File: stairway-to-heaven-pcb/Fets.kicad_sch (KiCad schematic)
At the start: 7 parts, among them J14 Conn_01x04_Male, Q40 FDN337N, Q41 FDN337N, Q42 FDN337N

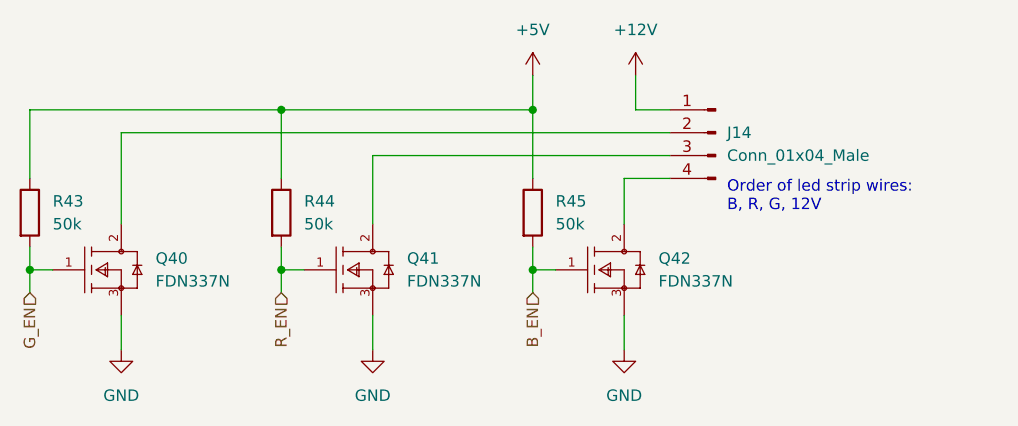
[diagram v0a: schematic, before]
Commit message: Change to 4 layer pcb. Routing leds done.
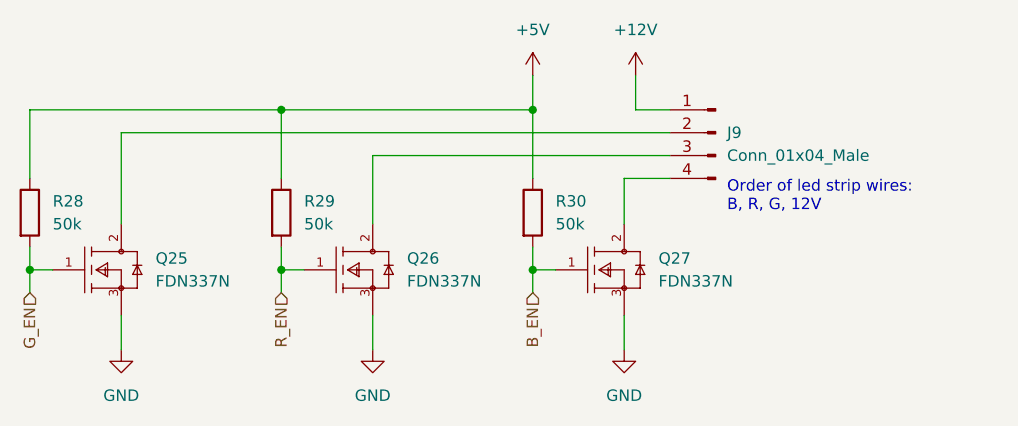
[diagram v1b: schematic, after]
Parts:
- renumbered J14 to J9, Q40 to Q25, Q41 to Q26, Q42 to Q27, R43 to R28, R44 to R29, R45 to R30
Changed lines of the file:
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@@
   (symbol (lib_id "Device:R") (at 96.52 99.06 0)
     (in_bom yes) (on_board yes) (fields_autoplaced)
-    (property "Reference" "R43" (id 0) (at 99.06 97.7899 0)
+    (property "Reference" "R28" (id 0) (at 99.06 97.7899 0)
       (effects (font (size 1.27 1.27)) (justify left))
     )
@@
   (symbol (lib_id "FDN337N:FDN337N") (at 96.52 105.41 0)
     (in_bom yes) (on_board yes) (fields_autoplaced)
-    (property "Reference" "Q40" (id 0) (at 110.49 104.1399 0)
+    (property "Reference" "Q25" (id 0) (at 110.49 104.1399 0)
       (effects (font (size 1.27 1.27)) (justify left))
     )
@@
   (symbol (lib_id "FDN337N:FDN337N") (at 152.4 105.41 0)
     (in_bom yes) (on_board yes) (fields_autoplaced)
-    (property "Reference" "Q42" (id 0) (at 166.37 104.1399 0)
+    (property "Reference" "Q27" (id 0) (at 166.37 104.1399 0)
       (effects (font (size 1.27 1.27)) (justify left))
     )
@@
   (symbol (lib_id "Connector:Conn_01x04_Male") (at 172.72 90.17 0) (mirror y)
     (in_bom yes) (on_board yes) (fields_autoplaced)
-    (property "Reference" "J14" (id 0) (at 173.99 90.1699 0)
+    (property "Reference" "J9" (id 0) (at 173.99 90.1699 0)
       (effects (font (size 1.27 1.27)) (justify right))
     )
@@
   (symbol (lib_id "FDN337N:FDN337N") (at 124.46 105.41 0)
     (in_bom yes) (on_board yes) (fields_autoplaced)
-    (property "Reference" "Q41" (id 0) (at 138.43 104.1399 0)
+    (property "Reference" "Q26" (id 0) (at 138.43 104.1399 0)
       (effects (font (size 1.27 1.27)) (justify left))
     )
@@
   (symbol (lib_id "Device:R") (at 152.4 99.06 0)
     (in_bom yes) (on_board yes) (fields_autoplaced)
-    (property "Reference" "R45" (id 0) (at 154.94 97.7899 0)
+    (property "Reference" "R30" (id 0) (at 154.94 97.7899 0)
       (effects (font (size 1.27 1.27)) (justify left))
     )
@@
   (symbol (lib_id "Device:R") (at 124.46 99.06 0)
     (in_bom yes) (on_board yes) (fields_autoplaced)
-    (property "Reference" "R44" (id 0) (at 127 97.7899 0)
-      (effects (font (size 1.27 1.27)) (justify left))
-    )
+    (property "Reference" "R29" (id 0) (at 127 97.7899 0)
+      (effects (font (size 1.27 1.27)) (justify left))
+    )

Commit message: PSU, again.. Stitching. Moved arduino nano.
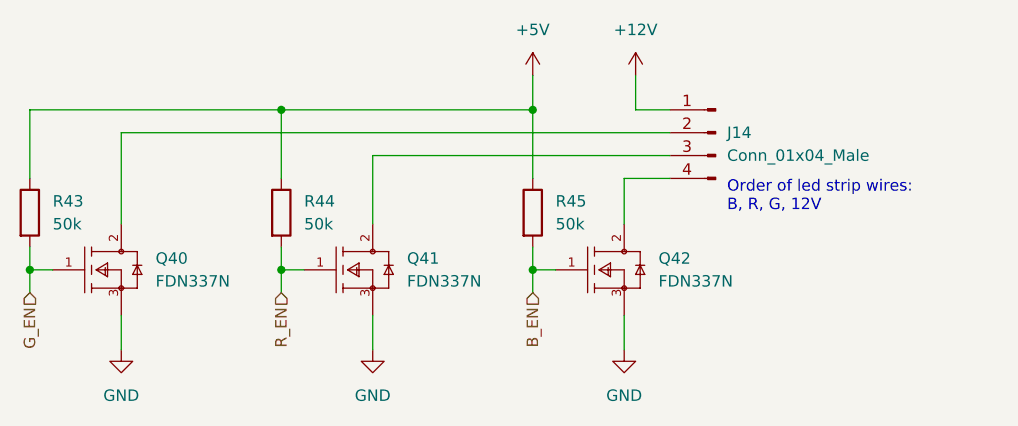
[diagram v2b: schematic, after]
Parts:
- renumbered J9 to J14, Q25 to Q40, Q26 to Q41, Q27 to Q42, R28 to R43, R29 to R44, R30 to R45
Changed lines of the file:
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@@
   (symbol (lib_id "Device:R") (at 96.52 99.06 0)
     (in_bom yes) (on_board yes) (fields_autoplaced)
-    (property "Reference" "R28" (id 0) (at 99.06 97.7899 0)
+    (property "Reference" "R43" (id 0) (at 99.06 97.7899 0)
       (effects (font (size 1.27 1.27)) (justify left))
     )
@@
   (symbol (lib_id "FDN337N:FDN337N") (at 96.52 105.41 0)
     (in_bom yes) (on_board yes) (fields_autoplaced)
-    (property "Reference" "Q25" (id 0) (at 110.49 104.1399 0)
+    (property "Reference" "Q40" (id 0) (at 110.49 104.1399 0)
       (effects (font (size 1.27 1.27)) (justify left))
     )
@@
   (symbol (lib_id "FDN337N:FDN337N") (at 152.4 105.41 0)
     (in_bom yes) (on_board yes) (fields_autoplaced)
-    (property "Reference" "Q27" (id 0) (at 166.37 104.1399 0)
+    (property "Reference" "Q42" (id 0) (at 166.37 104.1399 0)
       (effects (font (size 1.27 1.27)) (justify left))
     )
@@
   (symbol (lib_id "Connector:Conn_01x04_Male") (at 172.72 90.17 0) (mirror y)
     (in_bom yes) (on_board yes) (fields_autoplaced)
-    (property "Reference" "J9" (id 0) (at 173.99 90.1699 0)
+    (property "Reference" "J14" (id 0) (at 173.99 90.1699 0)
       (effects (font (size 1.27 1.27)) (justify right))
     )
@@
   (symbol (lib_id "FDN337N:FDN337N") (at 124.46 105.41 0)
     (in_bom yes) (on_board yes) (fields_autoplaced)
-    (property "Reference" "Q26" (id 0) (at 138.43 104.1399 0)
+    (property "Reference" "Q41" (id 0) (at 138.43 104.1399 0)
       (effects (font (size 1.27 1.27)) (justify left))
     )
@@
   (symbol (lib_id "Device:R") (at 152.4 99.06 0)
     (in_bom yes) (on_board yes) (fields_autoplaced)
-    (property "Reference" "R30" (id 0) (at 154.94 97.7899 0)
+    (property "Reference" "R45" (id 0) (at 154.94 97.7899 0)
       (effects (font (size 1.27 1.27)) (justify left))
     )
@@
   (symbol (lib_id "Device:R") (at 124.46 99.06 0)
     (in_bom yes) (on_board yes) (fields_autoplaced)
-    (property "Reference" "R29" (id 0) (at 127 97.7899 0)
-      (effects (font (size 1.27 1.27)) (justify left))
-    )
+    (property "Reference" "R44" (id 0) (at 127 97.7899 0)
+      (effects (font (size 1.27 1.27)) (justify left))
+    )
